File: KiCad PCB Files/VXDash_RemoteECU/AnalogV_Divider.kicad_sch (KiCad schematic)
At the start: 7 parts

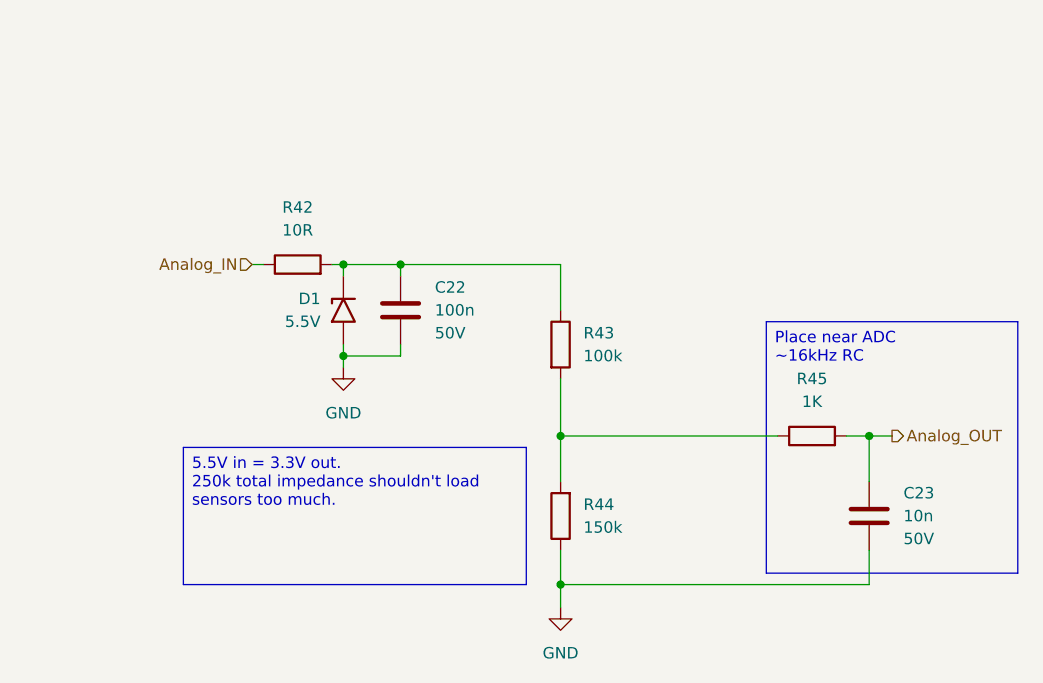
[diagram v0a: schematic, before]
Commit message: Started work on RemoteECU schematic
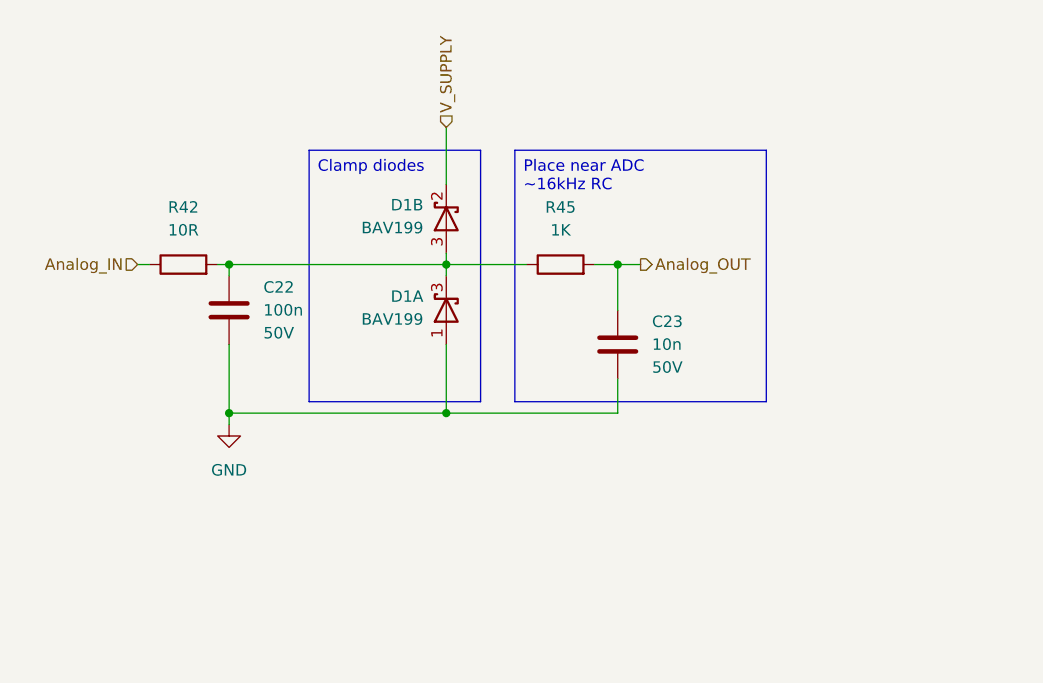
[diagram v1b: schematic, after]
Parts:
- removed D1: 5.5V, Diode_SMD:D_SOD-323_HandSoldering, symbol VXDash_diodes:TVS_Uni
- removed R43: 100k, Resistor_SMD:R_0805_2012Metric_Pad1.20x1.40mm_HandSolder, symbol VXDash_passives:Res
- removed R44: 150k, Resistor_SMD:R_0805_2012Metric_Pad1.20x1.40mm_HandSolder, symbol VXDash_passives:Res
- added D1: BAV199, Package_TO_SOT_SMD:SOT-23-3, symbol Device:D_Schottky_Dual_Series_AKC_Split
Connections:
- net GND: now also D1.1 (A)
- net at R45.1: now also C22.2, R42.2, D1.3 (K), D1.3 (K)
- new net V_SUPPLY: D1.2 (K)
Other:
- moved on the sheet: C22, C23, R42, R45
